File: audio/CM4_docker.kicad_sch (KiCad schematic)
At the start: 0 parts

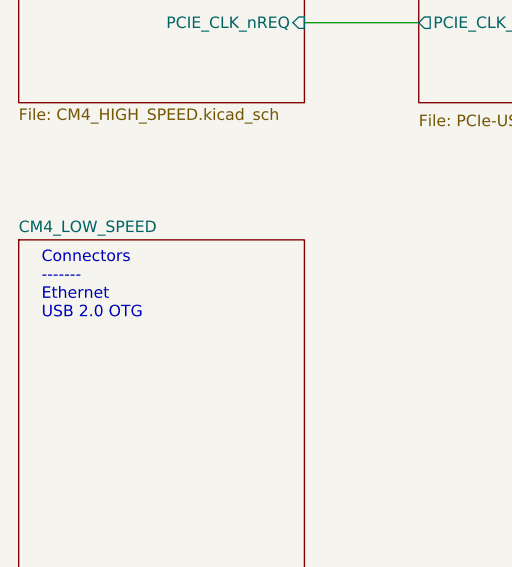
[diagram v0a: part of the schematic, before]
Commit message: .
.
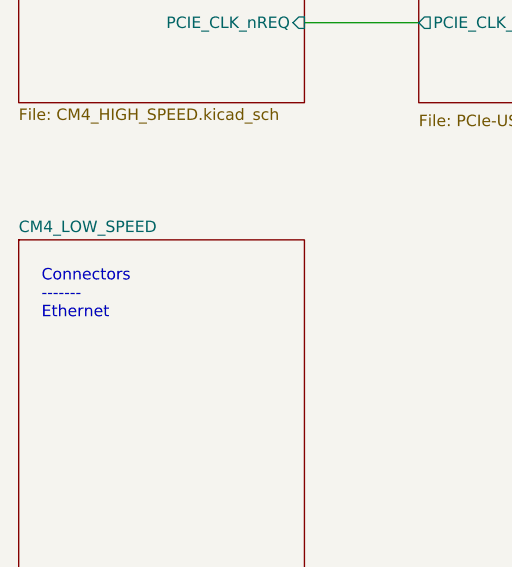
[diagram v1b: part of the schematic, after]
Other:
- note added: "Connectors ------- Ethernet"
- note removed: "Connectors ------- Ethernet USB 2.0 OTG"
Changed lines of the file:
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@@
     (effects (font (size 1.27 1.27)) (justify left bottom))
   )
-  (text "Connectors\n-------\nEthernet\nUSB 2.0 OTG" (at 40.64 102.87 0)
+  (text "Connectors\n-------\nEthernet" (at 40.64 102.87 0)
     (effects (font (size 1.27 1.27)) (justify left bottom))
   )

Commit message: .
.
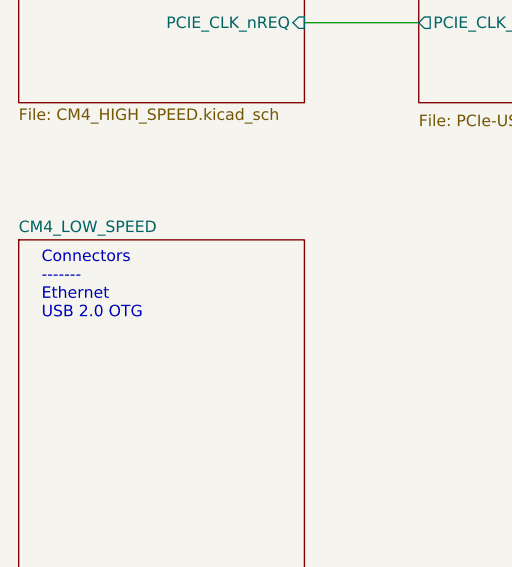
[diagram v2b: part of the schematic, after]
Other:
- note added: "Connectors ------- Ethernet USB 2.0 OTG"
- note removed: "Connectors ------- Ethernet"
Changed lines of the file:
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@@
     (effects (font (size 1.27 1.27)) (justify left bottom))
   )
-  (text "Connectors\n-------\nEthernet" (at 40.64 102.87 0)
+  (text "Connectors\n-------\nEthernet\nUSB 2.0 OTG" (at 40.64 102.87 0)
     (effects (font (size 1.27 1.27)) (justify left bottom))
   )
